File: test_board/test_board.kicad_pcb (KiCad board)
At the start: 4 copper layers, 68 parts, among them J101 Conn_01x02_Female, J102 Conn_01x04_Female, J103 Conn_01x04_Female, J104 Conn_01x01_Female, K301 KEYSW, K302 KEYSW, K303 KEYSW, K304 KEYSW, K305 KEYSW, K306 KEYSW, K307 KEYSW, K308 KEYSW, K309 KEYSW, K310 KEYSW, K311 KEYSW, K312 KEYSW, K313 KEYSW, K314 KEYSW, K315 KEYSW, K316 KEYSW, U201 WS2811, U202 WS2811, U203 WS2811, U204 WS2811, U205 WS2811, U206 WS2811, U207 WS2811, U208 WS2811, U209 WS2811, U210 WS2811, U211 WS2811, U212 WS2811, U213 WS2811, U214 WS2811, U215 WS2811, U216 WS2811

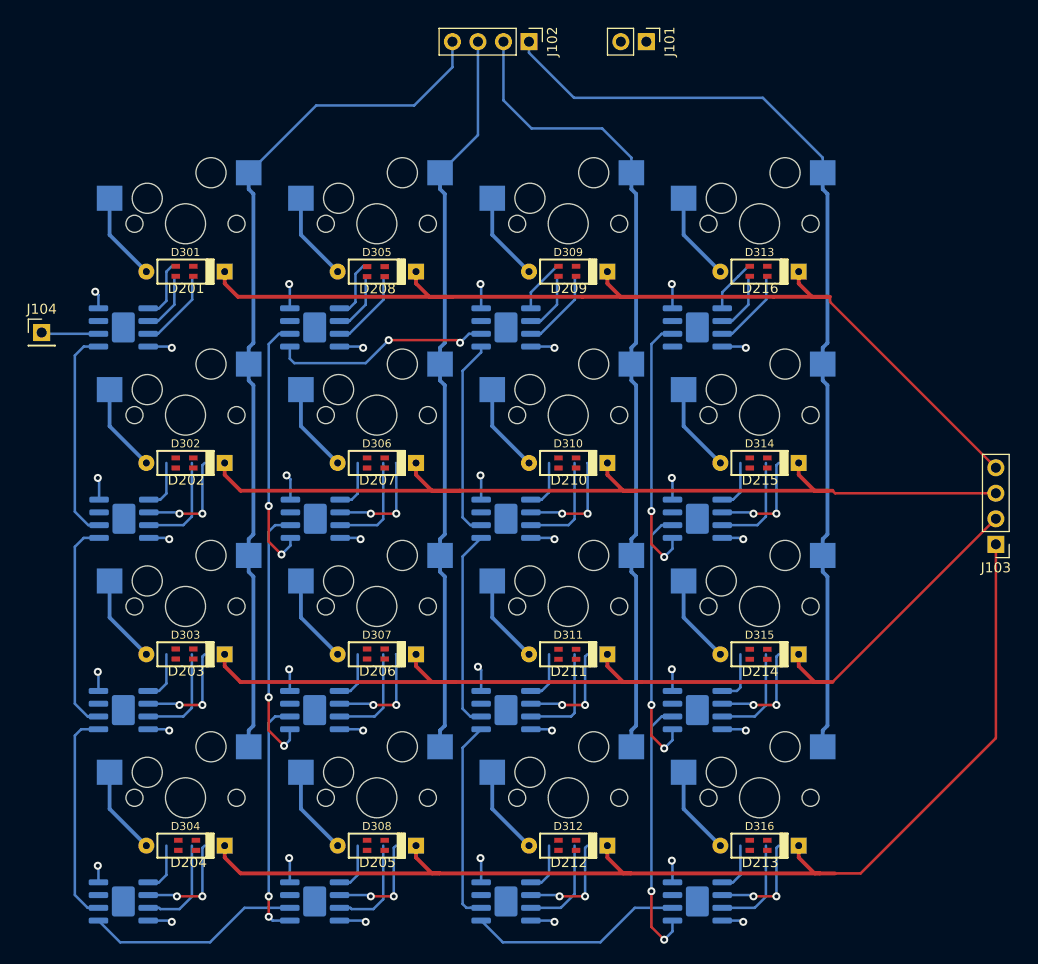
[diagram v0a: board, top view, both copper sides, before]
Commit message: example on pcb of how diodes might go
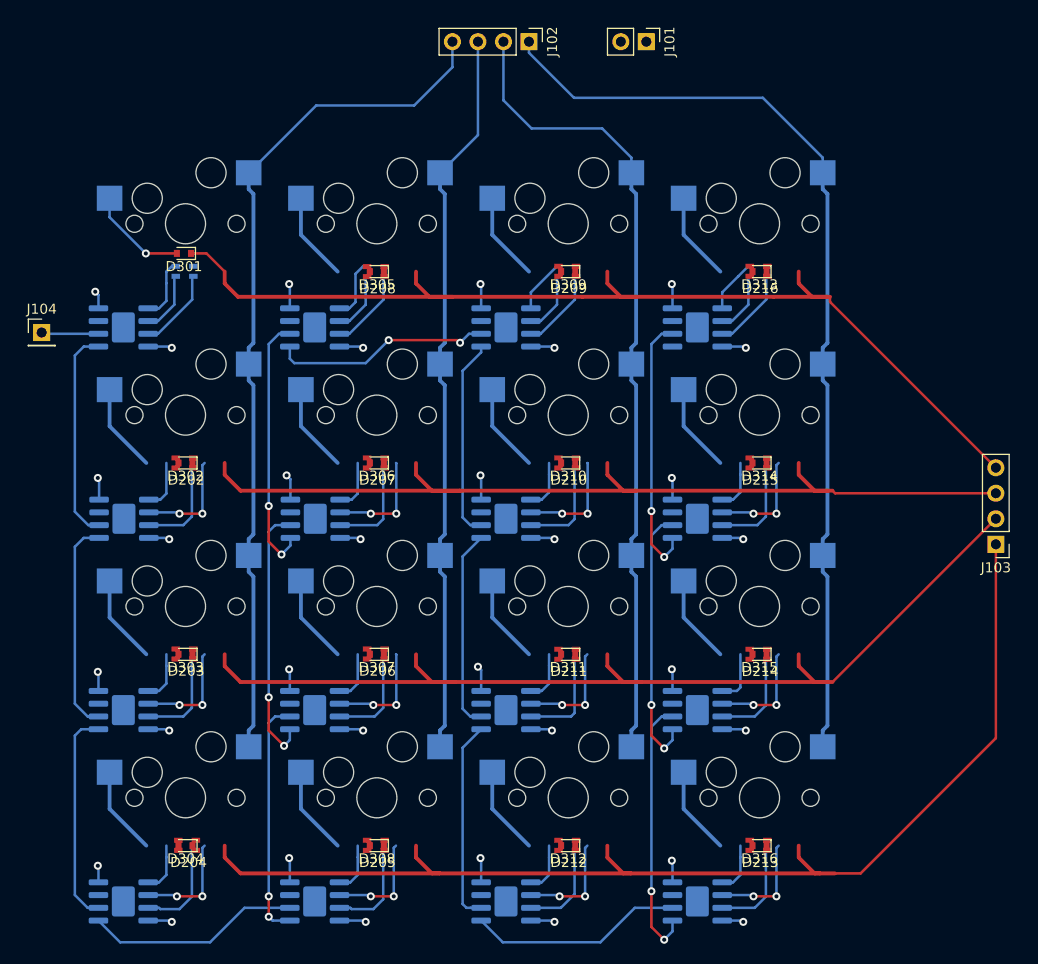
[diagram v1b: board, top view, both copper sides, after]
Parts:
- D201: moved to B.Cu
- D301, D302, D303, D304, D305, D306, D307, D308, D309, D310, D311, D312, D313, D314, D315, D316: footprint keyboard_parts:D_axial -> Diode_SMD:D_SOD-523
- moved D301 1.82 mm to (41.1, 59.4)
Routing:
- net /Row0: track 100.4 -> 104.4 mm
- net Net-(D301-Pad2): track 8.82 -> 10.1 mm, vias 0 -> 1
